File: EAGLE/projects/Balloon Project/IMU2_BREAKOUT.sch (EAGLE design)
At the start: 4 parts

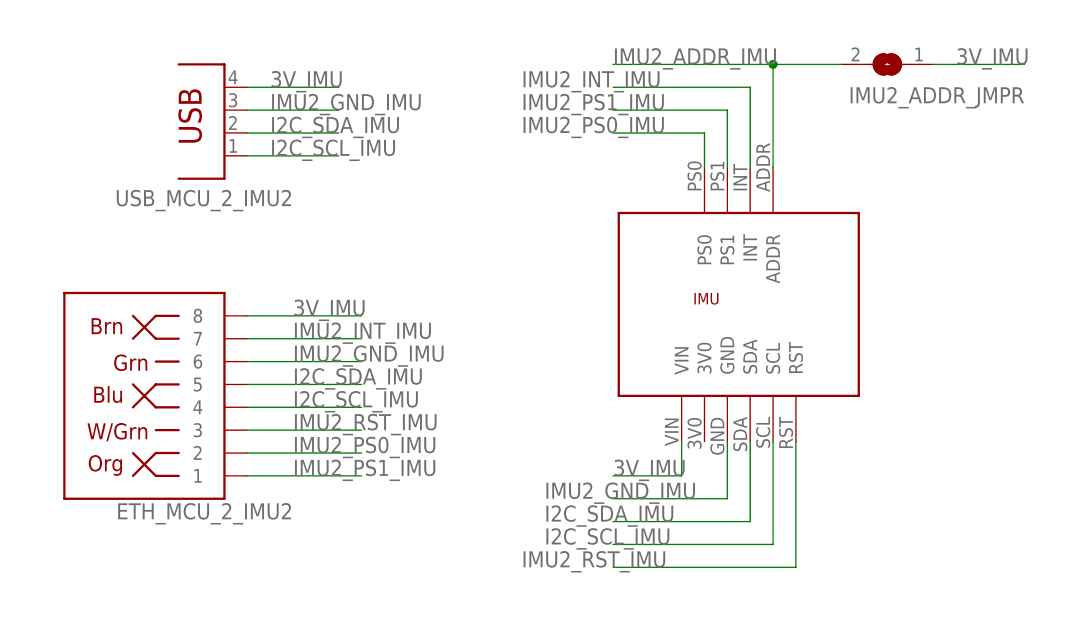
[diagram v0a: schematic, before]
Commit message: gerber files generated
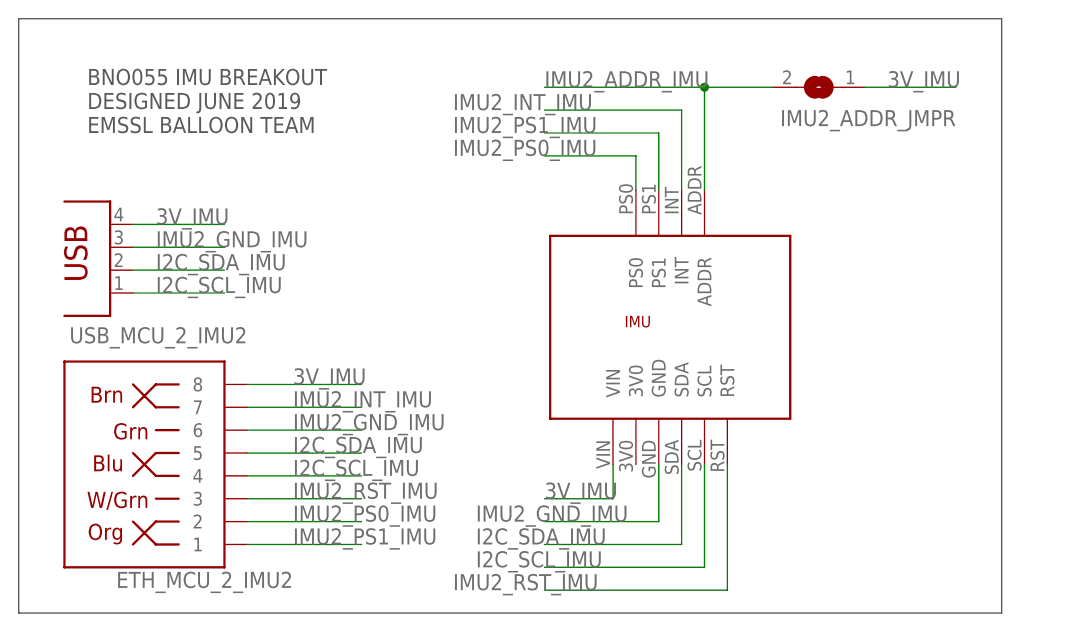
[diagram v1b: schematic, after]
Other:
- note added: "BNO055 IMU BREAKOUT DESIGNED JUNE 2019 EMSSL BALLOON TEAM"
- moved on the sheet: ETH_MCU_2_IMU2, IMU2_ADDR_JMPR, USB_MCU_2_IMU2
